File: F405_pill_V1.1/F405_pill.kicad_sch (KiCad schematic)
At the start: 42 parts, among them J1 Conn_01x04_Male, J2 Conn_01x04_Male, J4 TYPE-C-31-M-12, U1 STM32F405RGTx, U2 TCAN1051HDR, U3 LM1117-3.3, U4 STM32F405_pill, Y1 Crystal_GND24

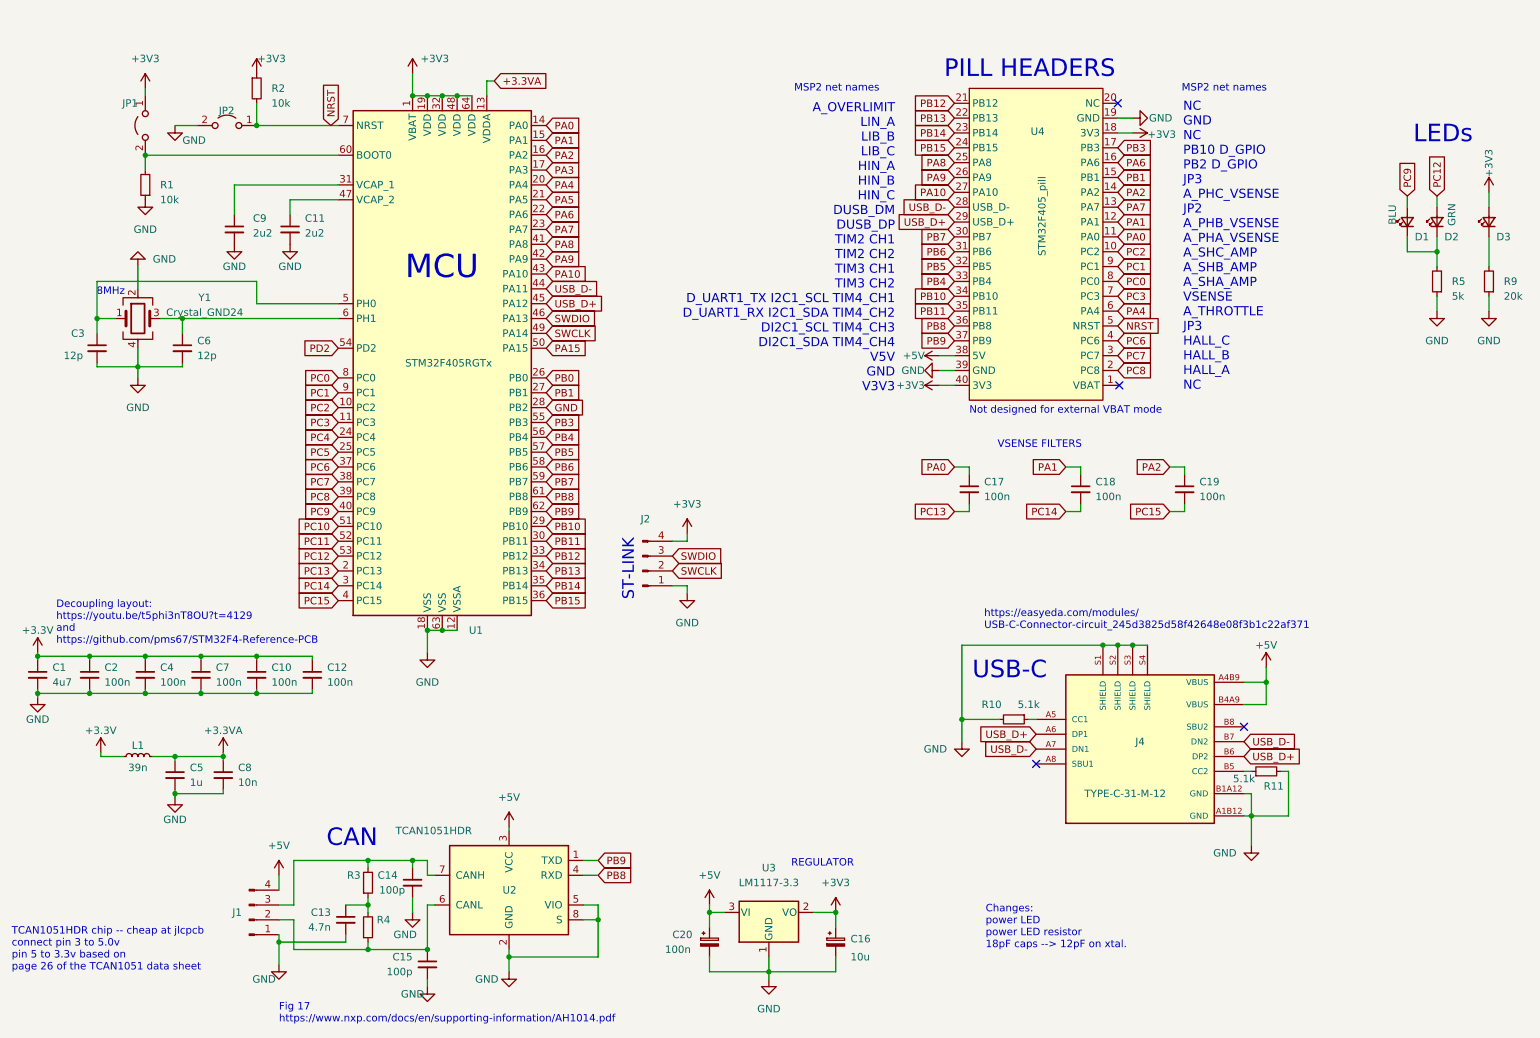
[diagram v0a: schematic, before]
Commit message: new work
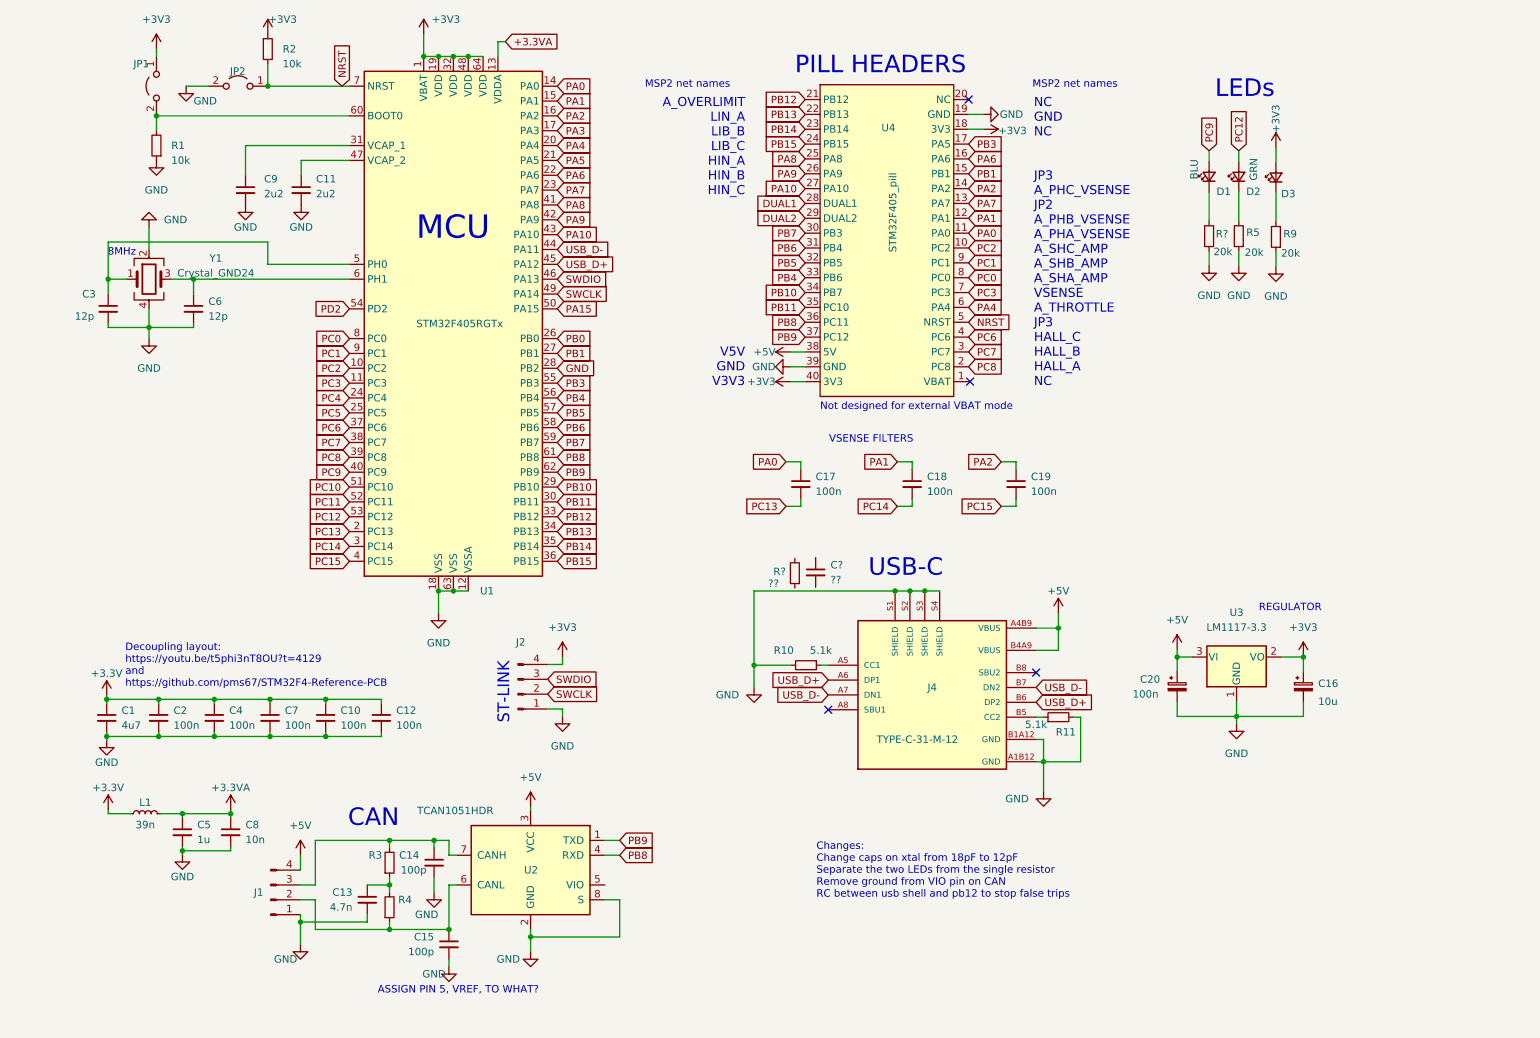
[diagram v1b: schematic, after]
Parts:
- added C?: ??, Capacitor_SMD:C_0402_1005Metric, symbol Device:C_Small
- added R?: ??, Resistor_SMD:R_0603_1608Metric, symbol Device:R_Small
- added R?: 20k, Resistor_SMD:R_0603_1608Metric, symbol Device:R_Small
- R5: value 5k -> 20k; LCSC C365441 -> C365403
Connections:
- net GND: now also R?.1; no longer U2.5 (VIO)
- net USB_D+: no longer U4.29 (USB_D+)
- net USB_D-: no longer U4.28 (USB_D-)
- net at D2.1 (K), R5.2: no longer D1.1 (K)
- new net: D1.1 (K), R?.2
- new net DUAL1: U4.28 (DUAL1)
- new net DUAL2: U4.29 (DUAL2)
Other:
- note added: "ASSIGN PIN 5, VREF, TO WHAT?"
- note added: "A_OVERLIMIT LIN_A LIB_B LIB_C HIN_A HIN_B HIN_C V5V GND V3V3"
- note added: "Changes: Change caps on xtal from 18pF to 12pF Separate the two LEDs from the single resistor Remove ground from VIO pin on CAN RC between usb shell and pb12 to stop false trips"
- note added: "NC GND NC JP3 A_PHC_VSENSE JP2 A_PHB_VSENSE A_PHA_VSENSE A_SHC_AMP A_SHB_AMP A_SHA_AMP VSENSE A_THROTTLE JP3 HALL_C HALL_B HALL_A NC"
- note removed: "A_OVERLIMIT LIN_A LIB_B LIB_C HIN_A HIN_B HIN_C DUSB_DM DUSB_DP TIM2 CH1 TIM2 CH2 TIM3 CH1 TIM3 CH2 D_UART1_TX I2C1_SCL TIM4_CH1 D_UART1_RX I2C1_SDA TIM4_CH2 DI2C1_SCL TIM4_CH3 DI2C1_SDA TIM4_CH4 V5V GND V3V3"
- note removed: "Changes: power LED power LED resistor 18pF caps --> 12pF on xtal."
- note removed: "Fig 17 https://www.nxp.com/docs/en/supporting-information/AH1014.pdf"
- note removed: "NC GND NC PB10 D_GPIO PB2 D_GPIO JP3 A_PHC_VSENSE JP2 A_PHB_VSENSE A_PHA_VSENSE A_SHC_AMP A_SHB_AMP A_SHA_AMP VSENSE A_THROTTLE JP3 HALL_C HALL_B HALL_A NC"
- note removed: "TCAN1051HDR chip -- cheap at jlcpcb connect pin 3 to 5.0v pin 5 to 3.3v based on page 26 of the TCAN1051 data sheet"
- note removed: "https://easyeda.com/modules/ USB-C-Connector-circuit_245d3825d58f42648e08f3b1c22af371"
- moved on the sheet: C1, C10, C11, C12, C13, C14, C15, C16, C17, C18, C19, C2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

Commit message: new notes
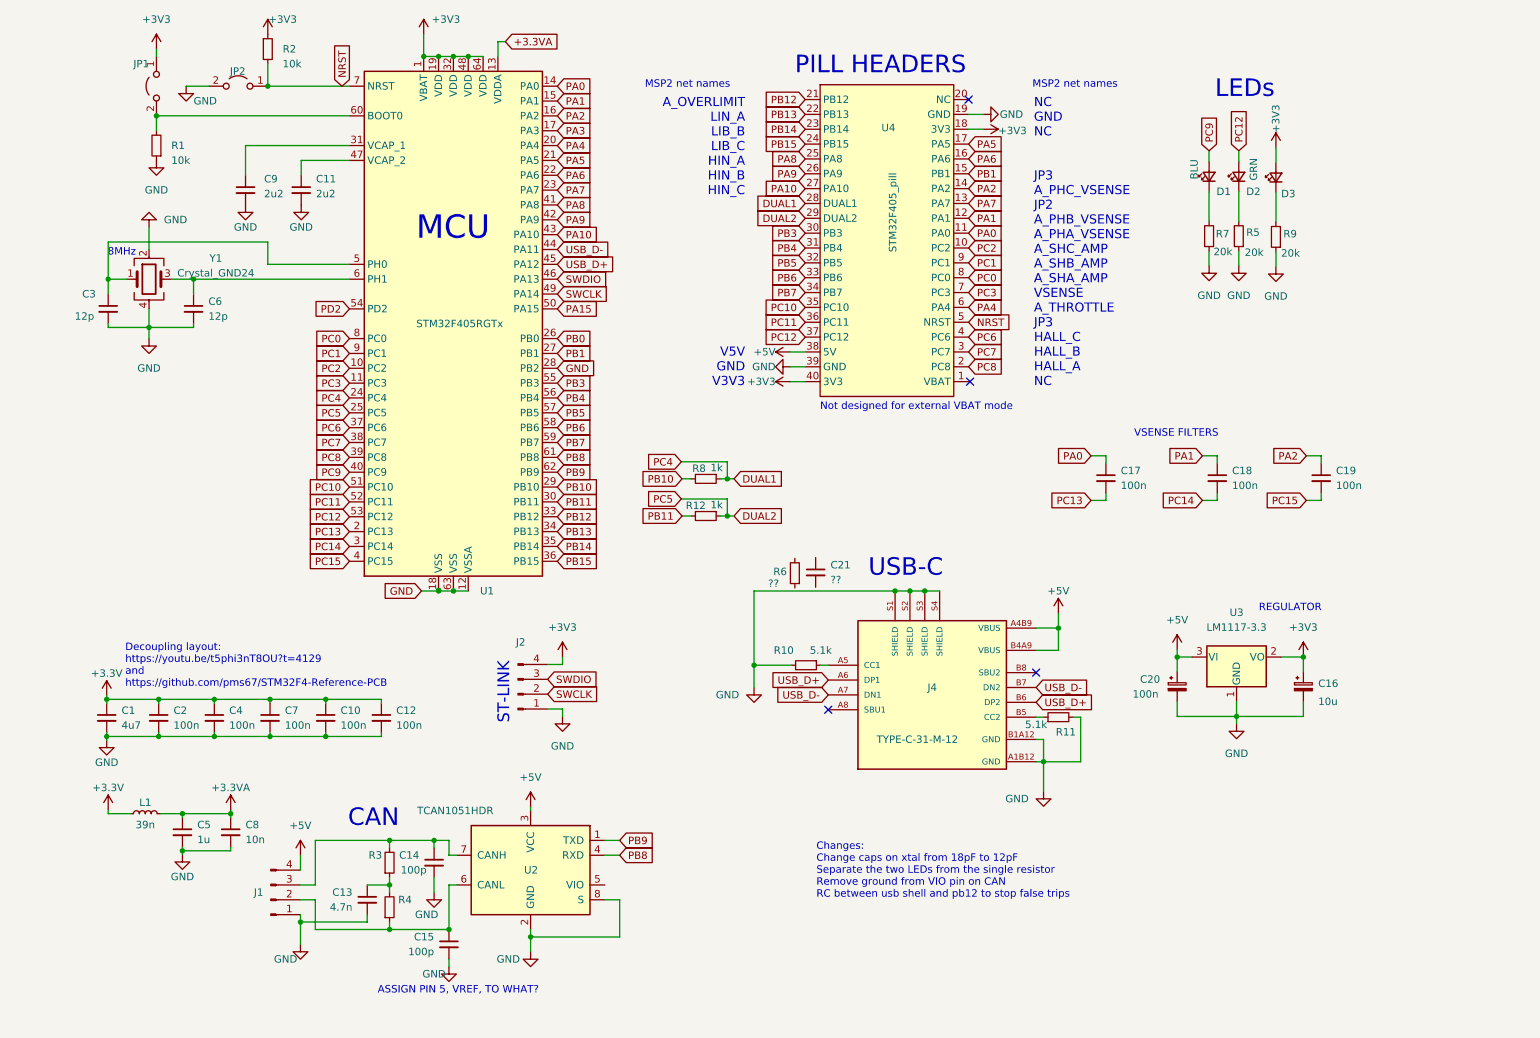
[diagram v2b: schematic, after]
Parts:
- added R12, R8: 1k, Resistor_SMD:R_0402_1005Metric, symbol Device:R_Small
- D3: footprint LED_SMD:LED_0603_1608Metric -> LED_SMD:LED_0402_1005Metric_Pad0.77x0.64mm_HandSolder
- R1, R2: footprint Resistor_SMD:R_0603_1608Metric -> Resistor_SMD:R_0402_1005Metric; LCSC C269701 -> (none)
- R10, R11: footprint Resistor_SMD:R_0603_1608Metric -> Resistor_SMD:R_0402_1005Metric; LCSC C365441 -> (none)
- R3, R4: footprint Resistor_SMD:R_0603_1608Metric -> Resistor_SMD:R_0402_1005Metric; LCSC C101133 -> (none)
- R5, R9: footprint Resistor_SMD:R_0603_1608Metric -> Resistor_SMD:R_0402_1005Metric; LCSC C365403 -> (none)
- R6: renamed from R?; footprint Resistor_SMD:R_0603_1608Metric -> Resistor_SMD:R_0402_1005Metric
- R7: renamed from R?; footprint Resistor_SMD:R_0603_1608Metric -> Resistor_SMD:R_0402_1005Metric; LCSC C365403 -> (none)
- gave numbers to parts that had none: 1
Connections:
- net PC4 is gone; now on net DUAL1: U1.24 (PC4)
- net PC5 is gone; now on net DUAL2: U1.25 (PC5)
- net DUAL1: now also R8.1
- net DUAL2: now also R12.1
- net PA5: now also U4.17 (PA5)
- net PB10: now also R8.2; no longer U4.34 (PB7)
- net PB11: now also R12.2; no longer U4.35 (PC10)
- net PB3: now also U4.30 (PB3); no longer U4.17 (PA5)
- net PB4: now also U4.31 (PB4); no longer U4.33 (PB6)
- net PB6: now also U4.33 (PB6); no longer U4.31 (PB4)
- net PB7: now also U4.34 (PB7); no longer U4.30 (PB3)
- net PB8: no longer U4.36 (PC11)
- net PB9: no longer U4.37 (PC12)
- net PC10: now also U4.35 (PC10)
- net PC11: now also U4.36 (PC11)
- net PC12: now also U4.37 (PC12)
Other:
- moved on the sheet: C17, C18, C19
